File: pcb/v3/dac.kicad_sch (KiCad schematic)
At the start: 62 parts, among them U14 CS43198, U15 CS43198, U16 OPA1622

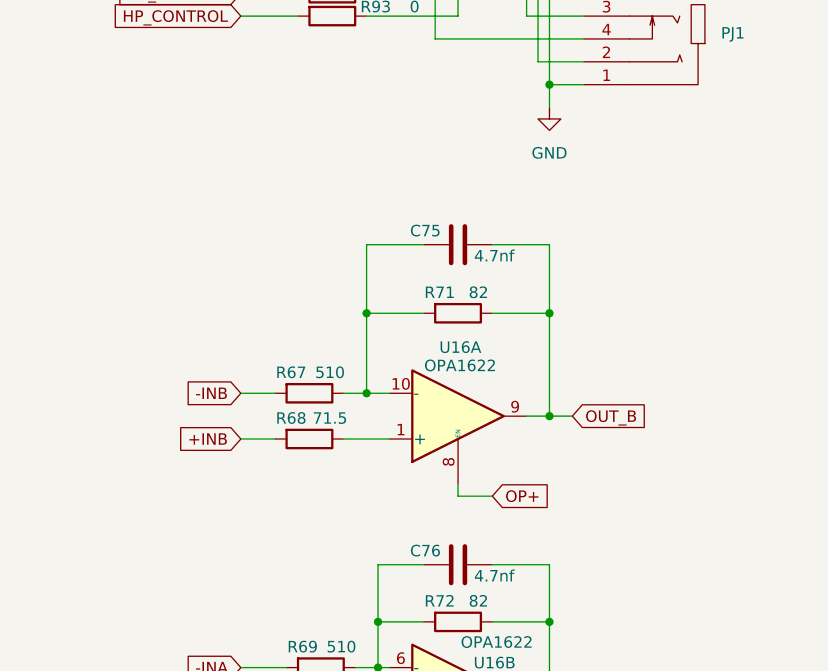
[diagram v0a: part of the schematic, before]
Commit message: up
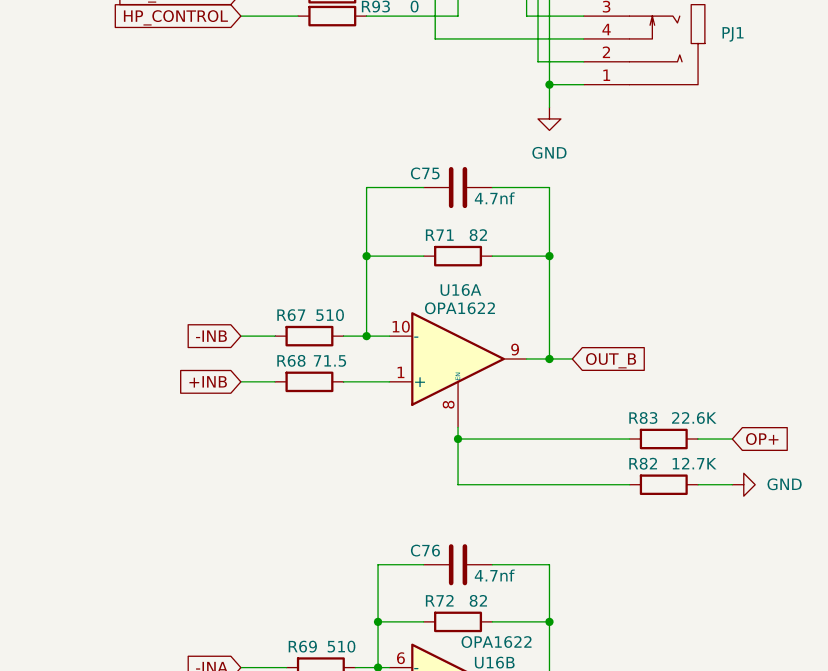
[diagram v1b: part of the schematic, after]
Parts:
- added R82: 12.7K, Resistor_SMD:R_0402_1005Metric_Pad0.72x0.64mm_HandSolder, symbol Device:R
- added R83: 22.6K, Resistor_SMD:R_0402_1005Metric_Pad0.72x0.64mm_HandSolder, symbol Device:R
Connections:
- net GND: now also R82.1
- net OP+: now also R83.1; no longer U16.8 (EN)
- new net: R82.2, R83.2, U16.8 (EN)
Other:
- moved on the sheet: C75, R67, R68, R71, U16A
